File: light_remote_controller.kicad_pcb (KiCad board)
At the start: 2 copper layers, 33 parts, among them J1 Conn_01x10_Female, J10 Screw_Terminal_01x02, J11 Screw_Terminal_01x02, J12 Conn_01x02_Female, J13 Screen, J2 Conn_01x03_Female, J3 Screw_Terminal_01x02, J4 Screw_Terminal_01x02, J5 Screw_Terminal_01x02, J6 Screw_Terminal_01x02, J7 Screw_Terminal_01x02, J8 Screw_Terminal_01x02, J9 Screw_Terminal_01x02, U1 NodeMCU_ESP12E, U2 WeMos_D1_mini, U3 PCF8574, U4 PCF8574

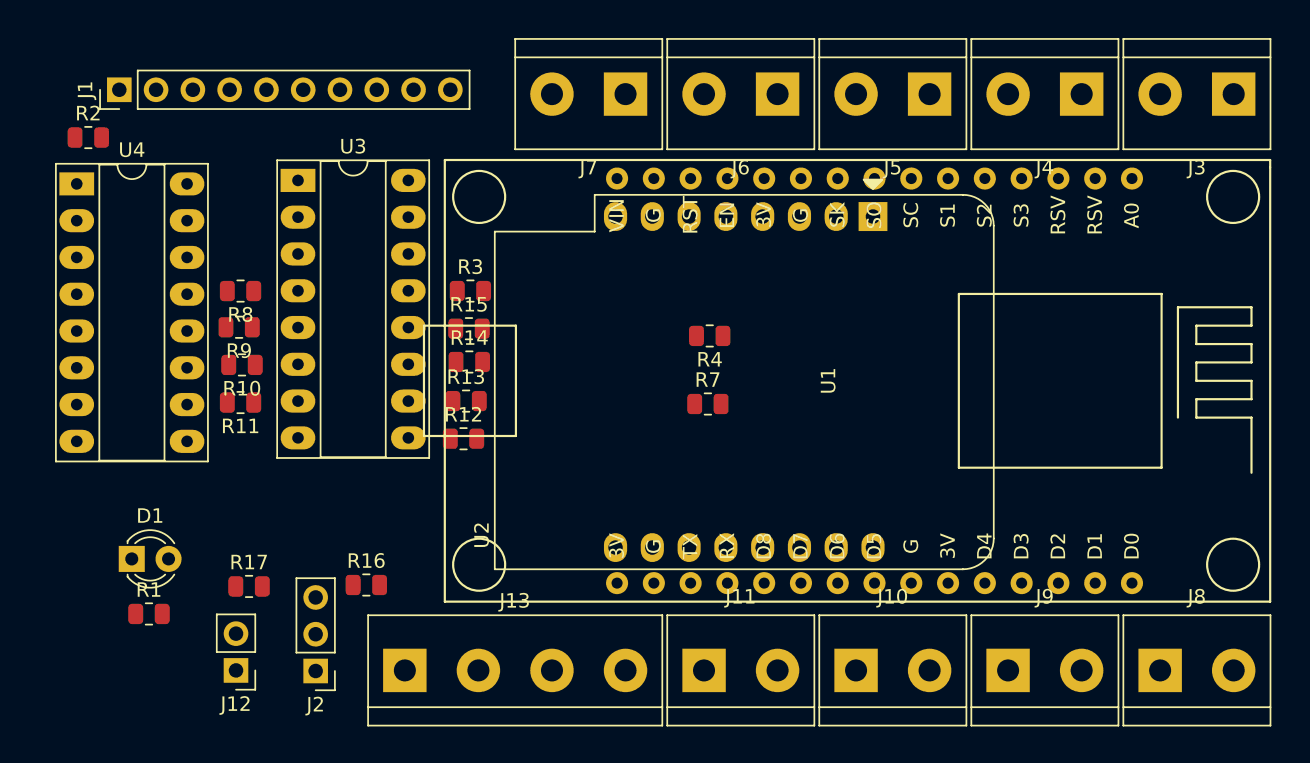
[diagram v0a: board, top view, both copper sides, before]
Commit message: Final version that went to production
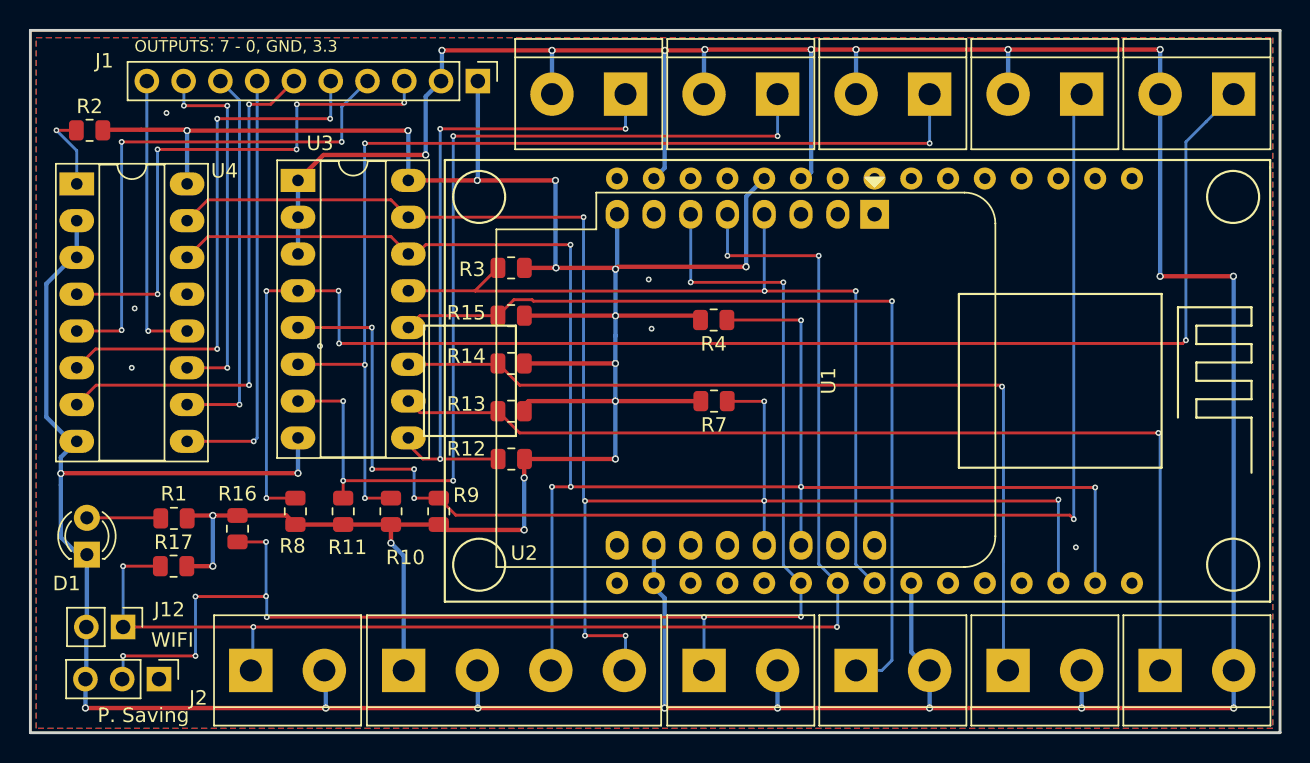
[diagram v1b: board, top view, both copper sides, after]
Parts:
- added J14: Screw_Terminal_01x02, TerminalBlock:TerminalBlock_bornier-2_P5.08mm, F.Cu at (188.9, 83.7)
- moved J1 24.8 mm to (204.6, 43.0), turned to -90 degrees
- moved R9 18.8 mm to (201.9, 72.7), turned to -90 degrees
- moved R8 15.7 mm to (192.0, 72.7), turned to -90 degrees
- moved R10 14.4 mm to (198.6, 72.7), turned to -90 degrees
- moved J2 10.8 mm to (182.6, 84.3), turned to -90 degrees
- moved R11 10.3 mm to (195.3, 72.7), turned to -90 degrees
- moved R16 9.71 mm to (188.0, 73.9), turned to 90 degrees
- moved J12 8.36 mm to (180.1, 80.7), turned to -90 degrees
- moved R1 6.82 mm to (183.6, 73.2), turned to 180 degrees
- moved R17 5.40 mm to (183.6, 76.5)
- moved R12 3.58 mm to (206.9, 69.1)
- moved R3 3.24 mm to (206.9, 55.9)
- moved R13 3.19 mm to (206.9, 65.8)
- moved D1 3.11 mm to (177.6, 75.7), turned to 90 degrees
- moved R15 3.05 mm to (206.9, 59.2)
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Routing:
- net GND: track 0.00 -> 320.0 mm, vias 0 -> 28
- net /+3V3: track 0.00 -> 175.1 mm, vias 0 -> 16
- net /I2C_SCL: track 0.00 -> 122.1 mm, vias 0 -> 6
- net /I2C_SDA: track 0.00 -> 113.6 mm, vias 0 -> 7
- net /BTN_0: track 0.00 -> 101.9 mm, vias 0 -> 5
- net /POWER_SAVING: track 0.00 -> 98.1 mm, vias 0 -> 10
- net /BTN_1: track 0.00 -> 95.5 mm, vias 0 -> 5
- net /BTN_WIFI: track 0.00 -> 94.5 mm, vias 0 -> 5
- net /BTN_2: track 0.00 -> 73.4 mm, vias 0 -> 4
- net /BTN_5: track 0.00 -> 69.2 mm, vias 0 -> 1
- net /BTN_3: track 0.00 -> 66.5 mm, vias 0 -> 5
- net /BTN_7: track 0.00 -> 61.8 mm, vias 0 -> 1
- net /BTN_6: track 0.00 -> 61.5 mm, vias 0 -> 1
- net /BTN_INT: track 0.00 -> 59.2 mm, vias 0 -> 2
- net /BTN_4: track 0.00 -> 45.1 mm, vias 0 -> 3
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- added copper zone on B.Cu, net GND
- added copper zone on F.Cu, net GND
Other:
- board outline added: 86.3 x 48.5 mm
- rule pad_to_mask_clearance: 0 -> 0.05
- board text added: "BTN_0"
- board text added: "BTN_1"
- board text added: "BTN_2"
- board text added: "BTN_3"
- board text added: "BTN_4"
- board text added: "BTN_5"
- board text added: "BTN_6"
- board text added: "BTN_7"
- board text added: "By Luis Pereira 20220605"
- board text added: "I2C (SDA, SCL, GND, 3V3)"
- board text added: "Light Remote"
- board text added: "OUTPUTS: 7 - 0, GND, 3.3"
- board text added: "P. Saving"
- board text added: "Pow. Saving"
- board text added: "V0.1"
- board text added: "WIFI"
